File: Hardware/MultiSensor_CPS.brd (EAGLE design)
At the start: 100 x 80 mm, 38 parts, among them U1 TCA9548APWR

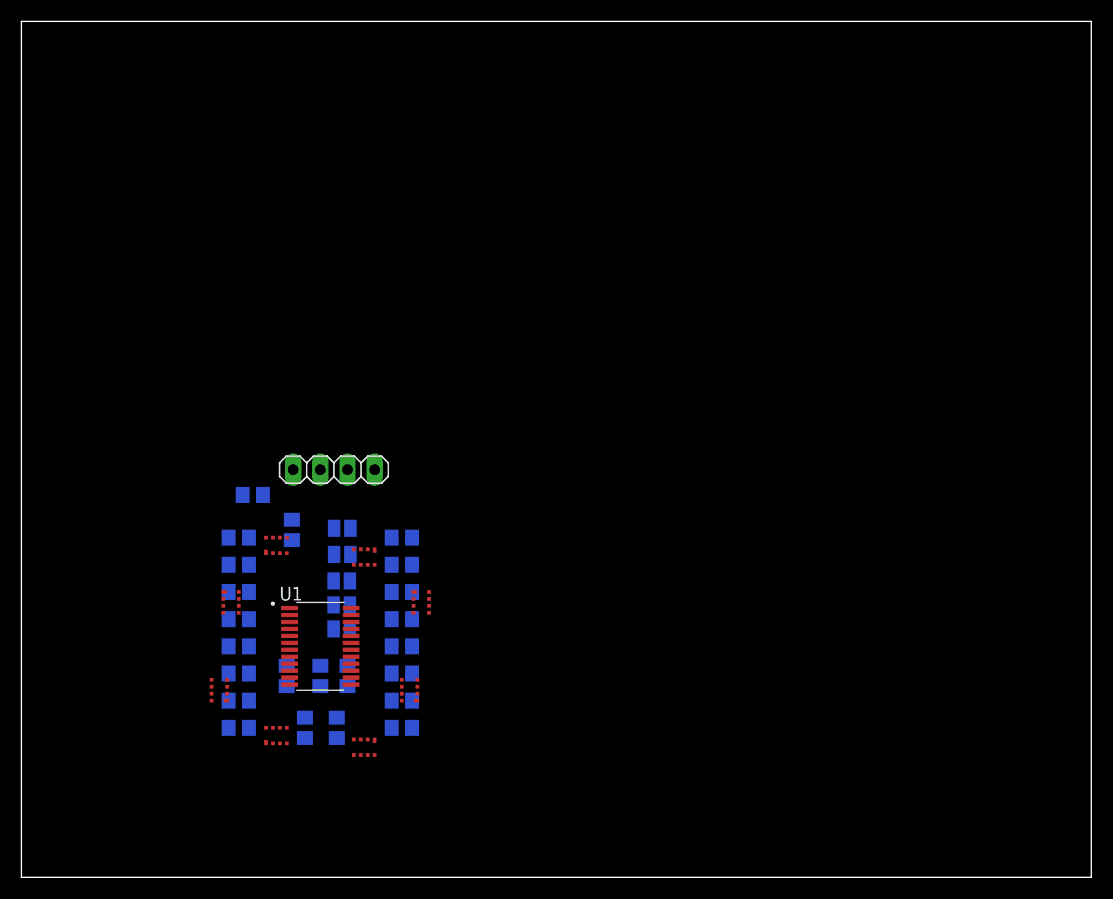
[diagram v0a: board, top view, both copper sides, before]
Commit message: prelim routing
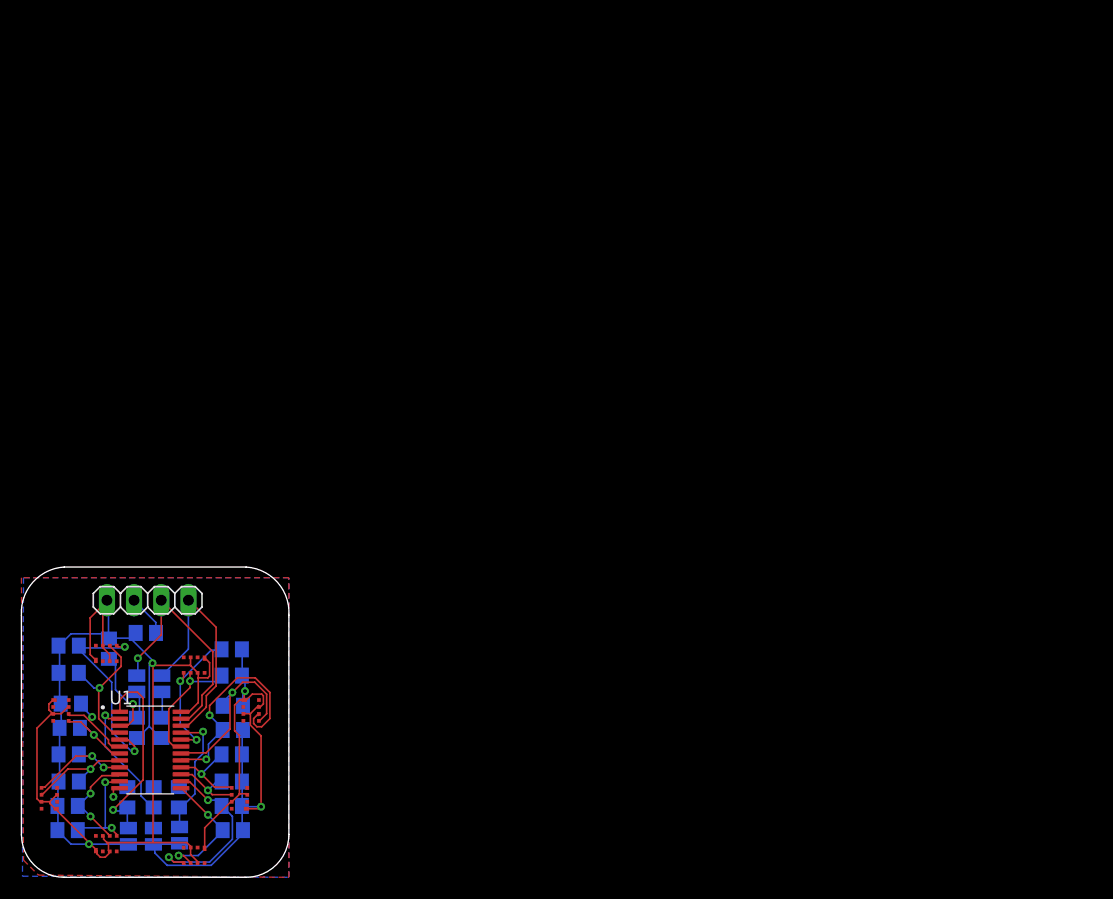
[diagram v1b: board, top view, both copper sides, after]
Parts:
- moved SJ1 31.1 mm to (10.0, 3.84), turned to 90 degrees
- moved SJ2 27.9 mm to (12.3, 3.84), turned to 90 degrees
- moved SJ3 24.5 mm to (14.8, 3.94), turned to 90 degrees
- moved SJ5 24.1 mm to (10.8, 18.1), turned to 90 degrees
- moved JP1 21.3 mm to (11.8, 25.9)
- moved SJ4 20.8 mm to (13.1, 18.1), turned to 90 degrees
- moved R16 20.5 mm to (19.7, 18.9)
- moved R14 20.4 mm to (19.8, 13.8)
- moved R17 20.4 mm to (8.18, 21.4)
- moved R3 20.3 mm to (4.52, 14.0)
- moved R7 20.1 mm to (4.32, 4.41)
- moved R10 19.9 mm to (19.8, 4.41)
- moved R20 19.4 mm to (14.7, 7.48), turned to 270 degrees
- moved R19 19.3 mm to (12.4, 7.48), turned to 270 degrees
- moved B1 18.8 mm to (4.42, 14.6)
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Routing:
- net VCC: track 0.00 -> 192.7 mm, vias 0 -> 4
- net SDA: track 0.00 -> 22.7 mm, vias 0 -> 1
- net SCL: track 0.00 -> 22.6 mm
- net SD6: track 0.00 -> 21.4 mm, vias 0 -> 2
- net SC0: track 0.00 -> 19.5 mm, vias 0 -> 2
- net A0: track 0.00 -> 18.8 mm, vias 0 -> 1
- net SC6: track 0.00 -> 17.6 mm, vias 0 -> 1
- net SC4: track 0.00 -> 17.0 mm, vias 0 -> 2
- net A1: track 0.00 -> 14.0 mm, vias 0 -> 1
- net SC7: track 0.00 -> 13.6 mm, vias 0 -> 2
- net SD0: track 0.00 -> 13.1 mm, vias 0 -> 1
- net SD4: track 0.00 -> 12.1 mm, vias 0 -> 2
- net A2: track 0.00 -> 12.1 mm, vias 0 -> 1
- net SD7: track 0.00 -> 11.8 mm, vias 0 -> 1
- net SC2: track 0.00 -> 10.3 mm, vias 0 -> 2
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- added copper zone on layer 1, net GND
- added copper zone on layer 16, net GND
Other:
- board size 100 x 80 mm -> 25 x 29 mm
